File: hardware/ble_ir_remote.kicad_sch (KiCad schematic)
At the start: 44 parts, among them J1 TYPE-C-31-M-12, J2 Debug connector, Q1 MMBT3904, U1 ESP32-C3-MINI-1-N4, U2 XC6206PxxxMR, U3 SRV05-4

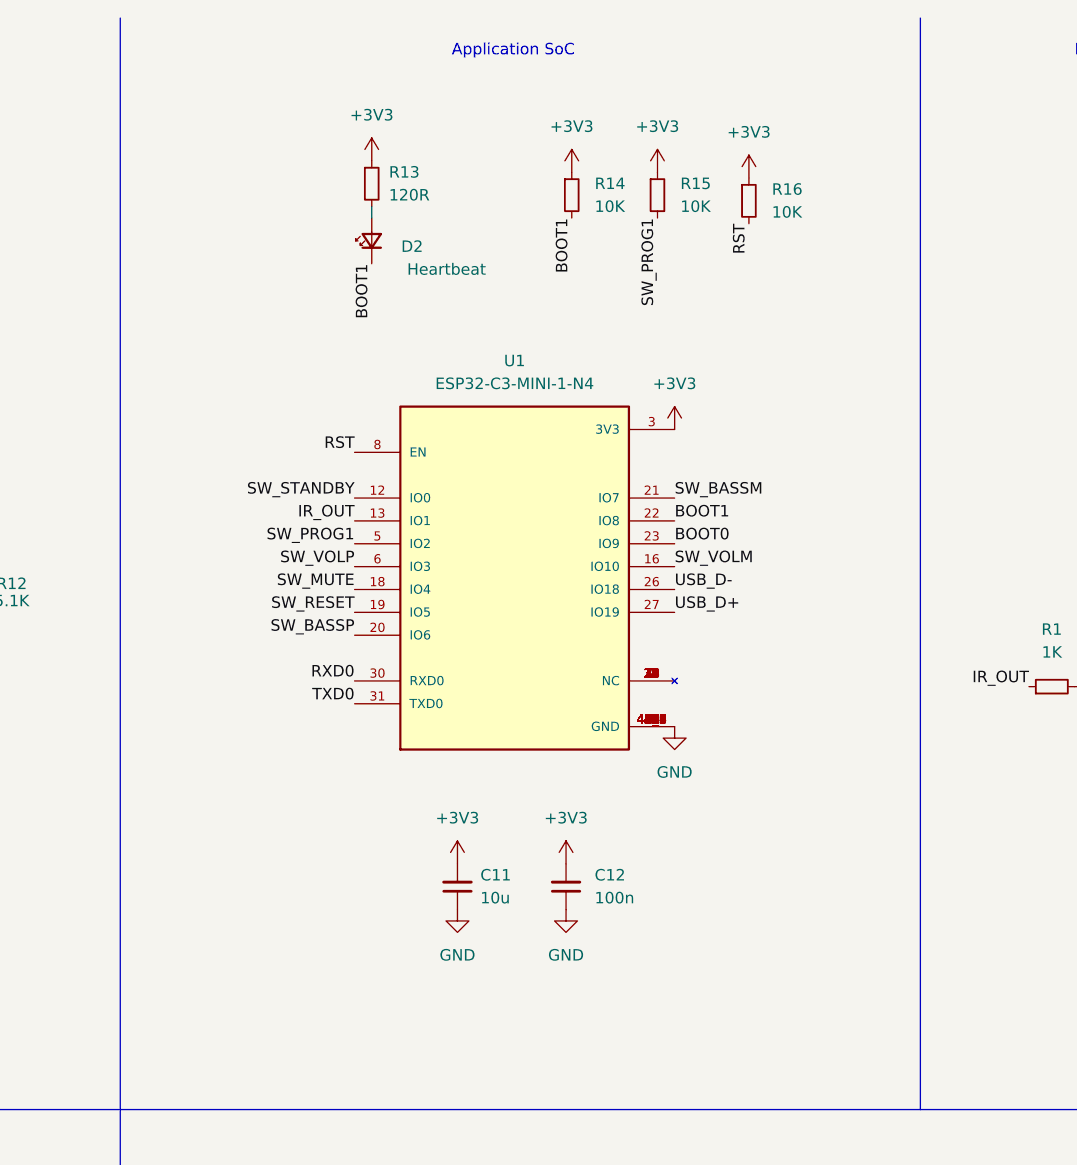
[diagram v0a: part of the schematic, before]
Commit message: cleanup
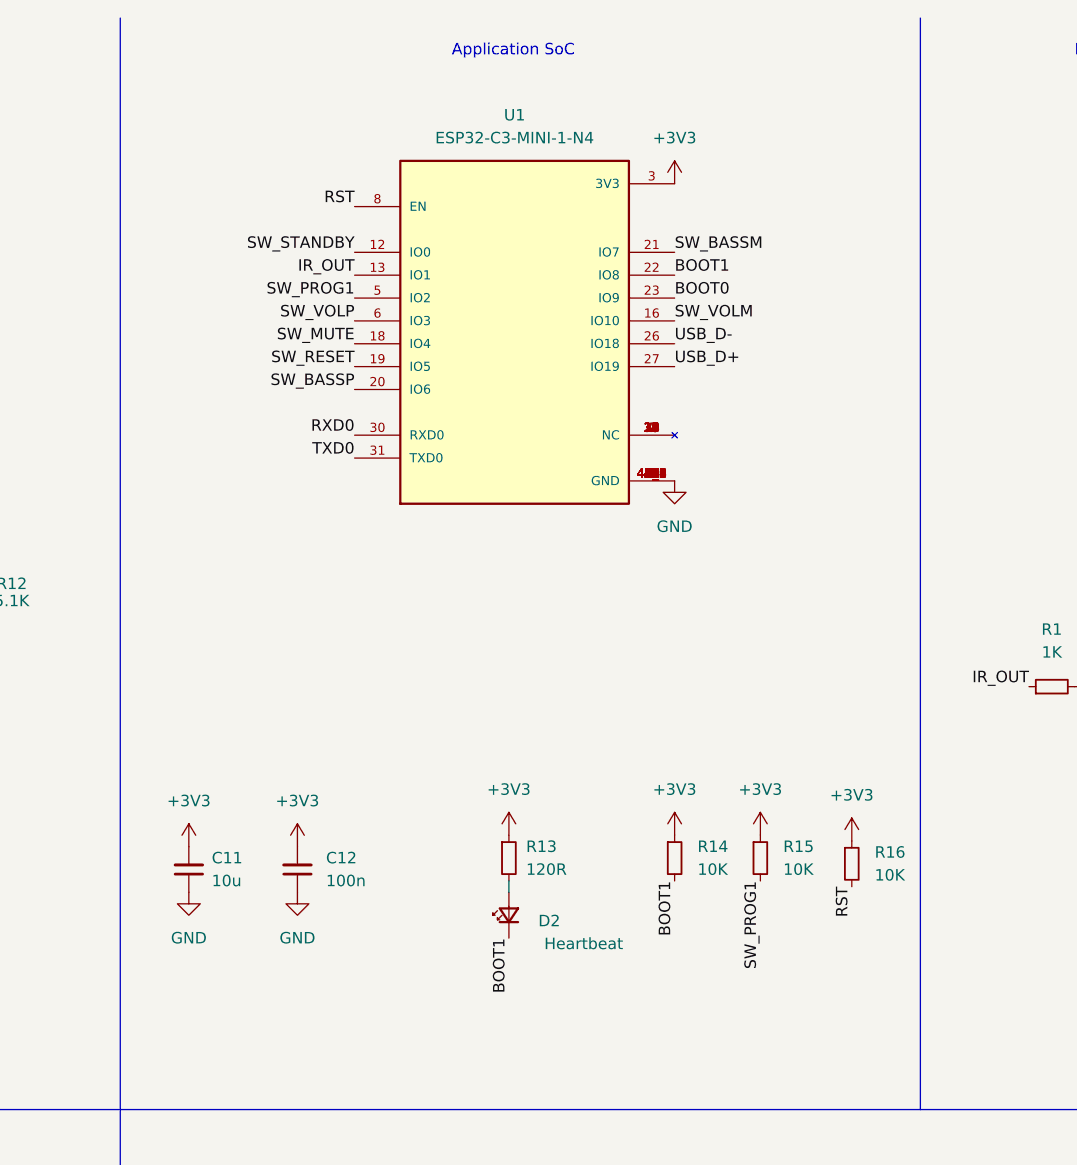
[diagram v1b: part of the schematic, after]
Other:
- moved on the sheet: C11, C12, D2, R13, R14, R15, R16, U1

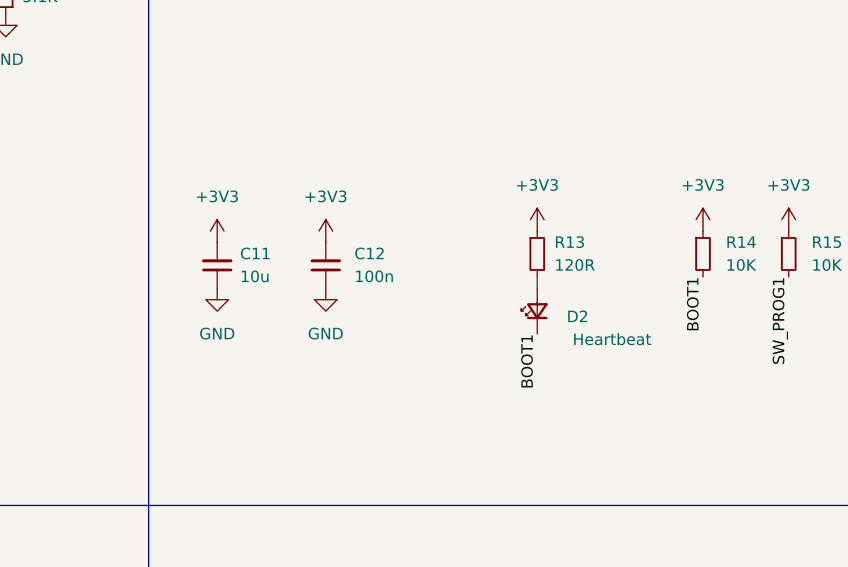
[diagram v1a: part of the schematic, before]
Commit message: cleanup
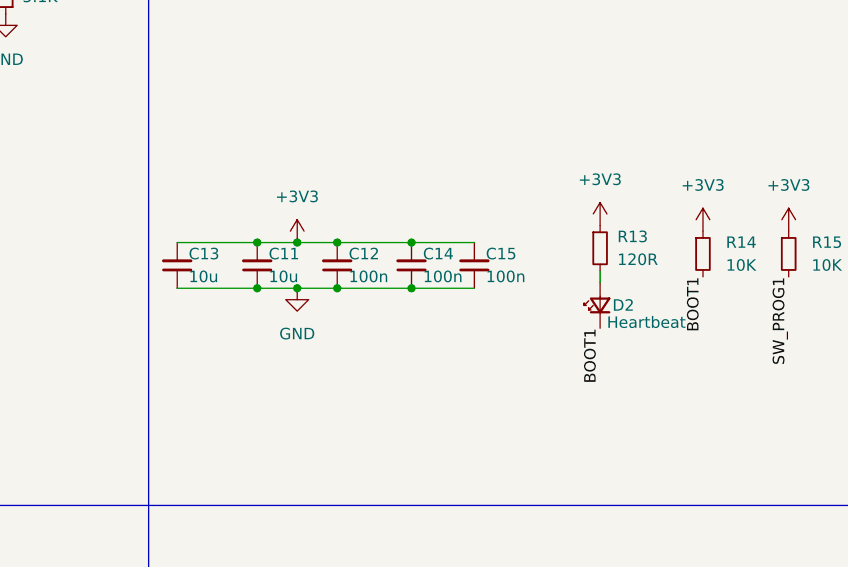
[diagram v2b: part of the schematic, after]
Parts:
- added C13: 10u, Capacitor_SMD:C_0603_1608Metric, symbol Device:C_Small
- added C14, C15: 100n, Capacitor_SMD:C_0603_1608Metric, symbol Device:C_Small
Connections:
- net +3V3: now also C13.2, C14.2, C15.2
- net GND: now also C13.1, C14.1, C15.1
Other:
- moved on the sheet: C11, C12, D2, R13
